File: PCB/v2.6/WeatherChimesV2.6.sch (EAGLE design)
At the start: 23 parts, among them U1 MS5803-02BA

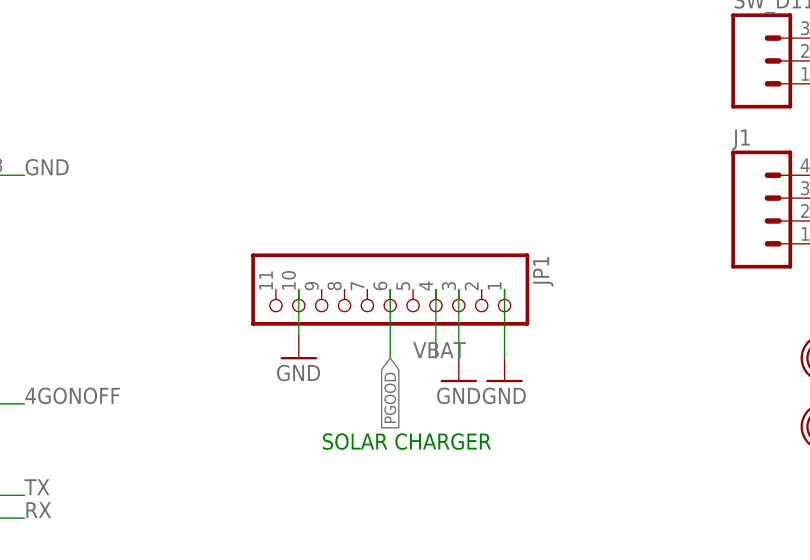
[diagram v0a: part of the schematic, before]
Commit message: Add files via upload
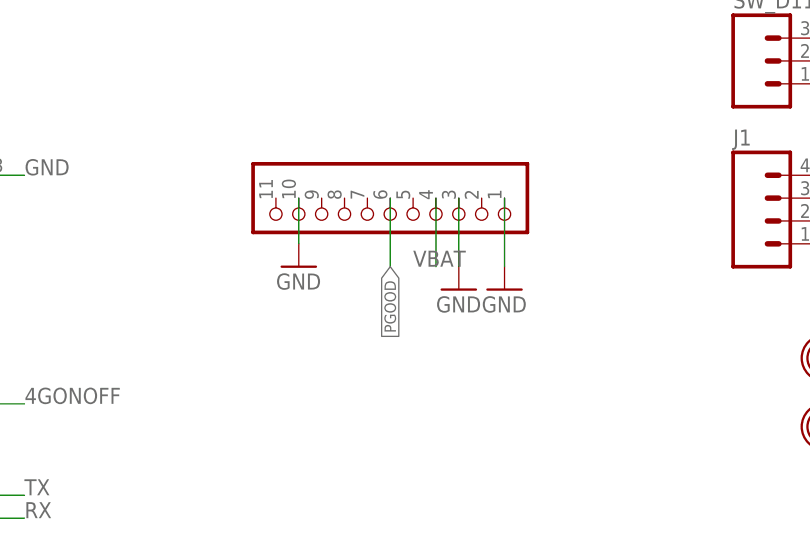
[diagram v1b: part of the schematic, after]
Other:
- note removed: "SOLAR CHARGER"
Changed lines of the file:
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@@
 <schematic_group name="MS580302BA"/>
 <schematic_group name="LTE_BOARD"/>
+<schematic_group name="SOLAR_CHARGER"/>
 </groups>
 <parts>
@@
 <sheet>
 <plain>
-<text x="83.82" y="-22.86" size="1.778" layer="91">SOLAR CHARGER</text>
 </plain>
 <instances>
@@
 <instance part="U$4" gate="G$1" x="139.7" y="-20.32" smashed="yes"/>
 <instance part="U$5" gate="G$1" x="147.32" y="-20.32" smashed="yes"/>
-<instance part="GND1" gate="1" x="81.28" y="-12.7" smashed="yes">
-<attribute name="VALUE" x="78.74" y="-15.24" size="1.778" layer="96"/>
-</instance>
-<instance part="JP1" gate="G$1" x="91.44" y="-7.62" smashed="yes" rot="R270">
-<attribute name="NAME" x="107.315" y="-1.27" size="1.778" layer="95" rot="R270"/>
-<attribute name="VALUE" x="73.66" y="-1.27" size="1.778" layer="96" rot="R270"/>
-</instance>
-<instance part="GND2" gate="1" x="104.14" y="-15.24" smashed="yes">
-<attribute name="VALUE" x="101.6" y="-17.78" size="1.778" layer="96"/>
-</instance>
-<instance part="GND3" gate="1" x="99.06" y="-15.24" smashed="yes">
-<attribute name="VALUE" x="96.52" y="-17.78" size="1.778" layer="96"/>
+<instance part="GND1" gate="1" x="81.28" y="-2.54" smashed="yes" grouprefs="SOLAR_CHARGER">
+<attribute name="VALUE" x="78.74" y="-5.08" size="1.778" layer="96"/>
+</instance>
+<instance part="JP1" gate="G$1" x="91.44" y="2.54" smashed="yes" rot="R270" grouprefs="SOLAR_CHARGER">
+<attribute name="VALUE" x="73.66" y="8.89" size="1.778" layer="96" rot="R270"/>
+</instance>
+<instance part="GND2" gate="1" x="104.14" y="-5.08" smashed="yes" grouprefs="SOLAR_CHARGER">
+<attribute name="VALUE" x="101.6" y="-7.62" size="1.778" layer="96"/>
+</instance>
+<instance part="GND3" gate="1" x="99.06" y="-5.08" smashed="yes" grouprefs="SOLAR_CHARGER">
+<attribute name="VALUE" x="96.52" y="-7.62" size="1.778" layer="96"/>
 </instance>
 <instance part="GND4" gate="1" x="147.32" y="30.48" smashed="yes" rot="R180">
@@
 </segment>
 <segment>
-<wire x1="81.28" y1="-5.08" x2="81.28" y2="-10.16" width="0.1524" layer="91"/>
+<wire x1="81.28" y1="5.08" x2="81.28" y2="0" width="0.1524" layer="91" grouprefs="SOLAR_CHARGER"/>
 <pinref part="GND1" gate="1" pin="GND"/>
 <pinref part="JP1" gate="G$1" pin="10"/>
@@
 <segment>
 <pinref part="GND2" gate="1" pin="GND"/>
-<wire x1="104.14" y1="-5.08" x2="104.14" y2="-12.7" width="0.1524" layer="91"/>
+<wire x1="104.14" y1="5.08" x2="104.14" y2="-2.54" width="0.1524" layer="91" grouprefs="SOLAR_CHARGER"/>
 <pinref part="JP1" gate="G$1" pin="1"/>
 </segment>
 <segment>
 <pinref part="GND3" gate="1" pin="GND"/>
-<wire x1="99.06" y1="-5.08" x2="99.06" y2="-12.7" width="0.1524" layer="91"/>
+<wire x1="99.06" y1="5.08" x2="99.06" y2="-2.54" width="0.1524" layer="91" grouprefs="SOLAR_CHARGER"/>
 <pinref part="JP1" gate="G$1" pin="3"/>
 </segment>
@@
 <segment>
 <pinref part="JP1" gate="G$1" pin="4"/>
-<wire x1="96.52" y1="-5.08" x2="96.52" y2="-12.7" width="0.1524" layer="91"/>
-<label x="93.98" y="-12.7" size="1.778" layer="95"/>
+<wire x1="96.52" y1="5.08" x2="96.52" y2="-2.54" width="0.1524" layer="91" grouprefs="SOLAR_CHARGER"/>
+<label x="93.98" y="-2.54" size="1.778" layer="95" grouprefs="SOLAR_CHARGER"/>
 </segment>
 <segment>
@@
 <segment>
 <pinref part="JP1" gate="G$1" pin="6"/>
-<wire x1="91.44" y1="-5.08" x2="91.44" y2="-12.7" width="0.1524" layer="91"/>
-<label x="91.44" y="-12.7" size="1.27" layer="95" rot="R270" xref="yes"/>
-</segment>
-<segment>
+<wire x1="91.44" y1="5.08" x2="91.44" y2="-2.54" width="0.1524" layer="91" grouprefs="SOLAR_CHARGER"/>
+<label x="91.44" y="-2.54" size="1.27" layer="95" rot="R270" xref="yes" grouprefs="SOLAR_CHARGER"/>
+</segment>
+<segment>
